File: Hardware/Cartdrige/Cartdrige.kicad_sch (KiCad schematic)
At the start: 3 parts, among them J2 PORT1, U1 28C256

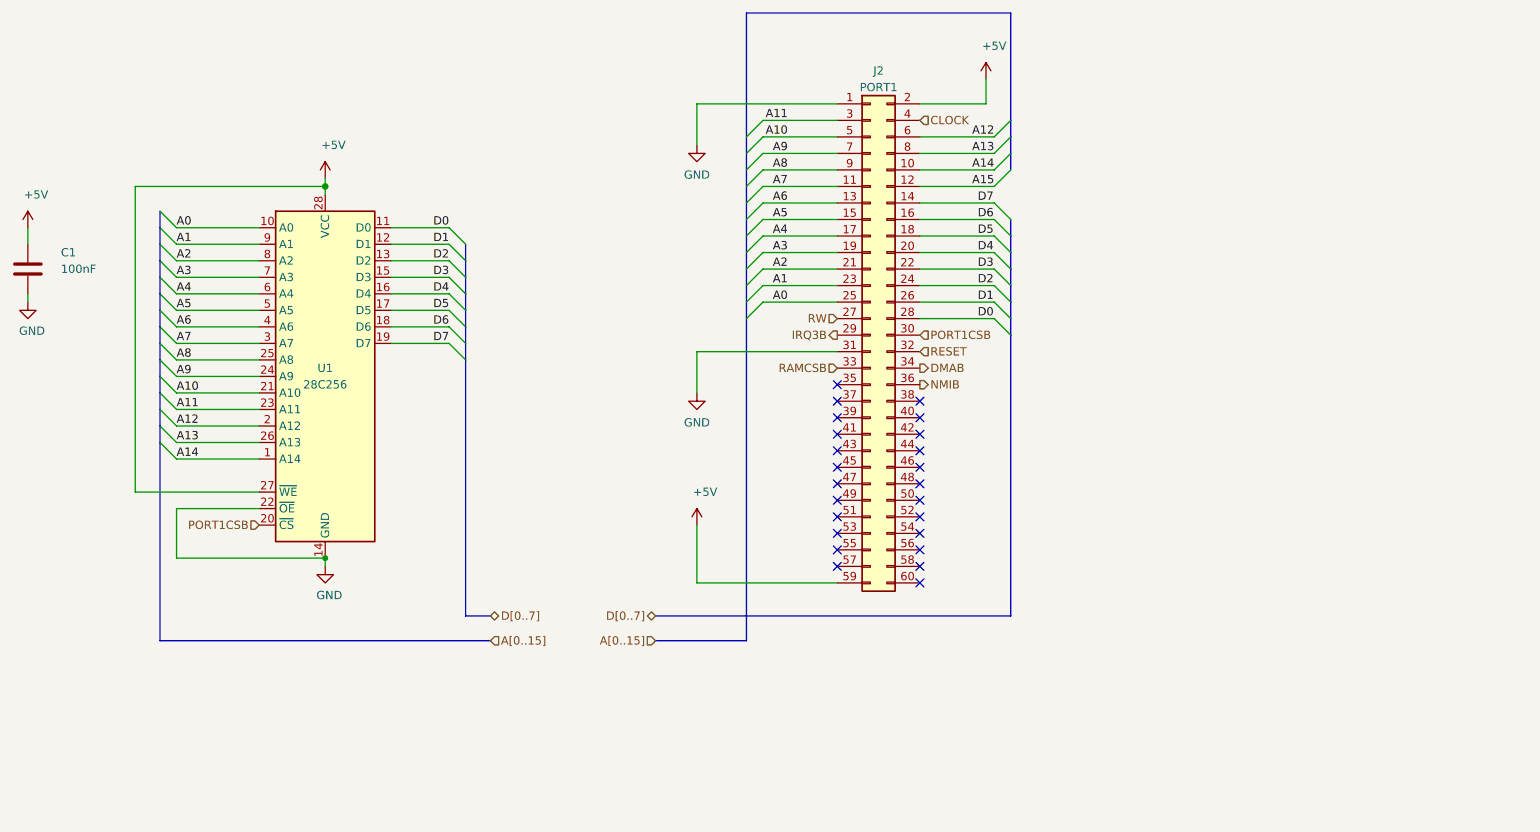
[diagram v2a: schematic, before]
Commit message: A lot of new hardware
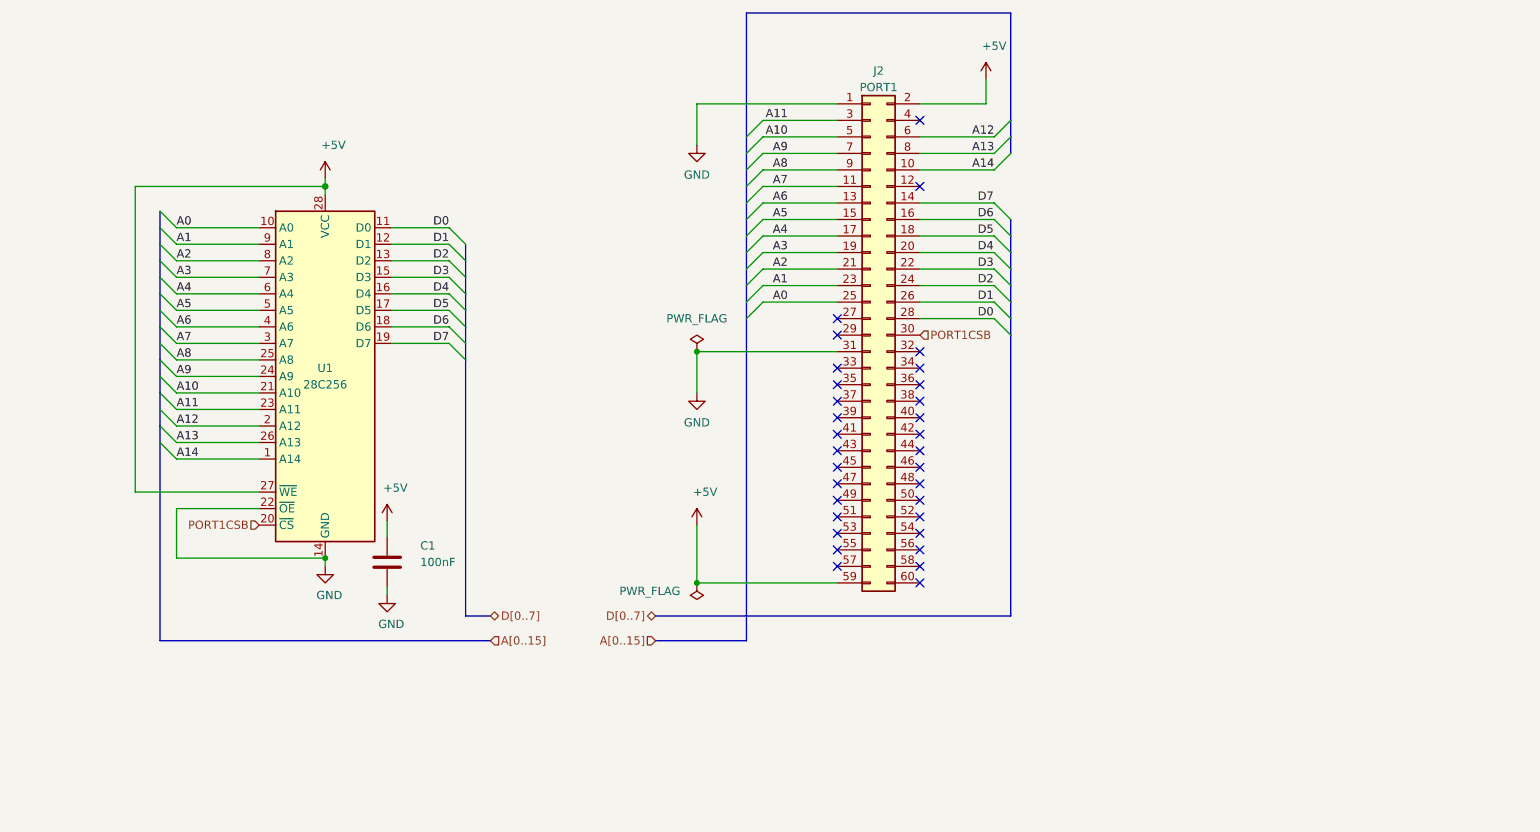
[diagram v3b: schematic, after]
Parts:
- J2: footprint NESConnector:NES_PCBEdge -> Connector_NES:NES_PCBEdge
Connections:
- net A15: no longer names the net of J2.12 (Pin_12)
- net CLOCK: no longer names the net of J2.4 (Pin_4)
- net DMAB: no longer names the net of J2.34 (Pin_34)
- net IRQ3B: no longer names the net of J2.29 (Pin_29)
- net NMIB: no longer names the net of J2.36 (Pin_36)
- net RAMCSB: no longer names the net of J2.33 (Pin_33)
- net RESET: no longer names the net of J2.32 (Pin_32)
- net RW: no longer names the net of J2.27 (Pin_27)
- no-connect marks 24 -> 32
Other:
- moved on the sheet: C1
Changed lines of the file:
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@@
   (junction (at 68.58 100.33) (diameter 0) (color 0 0 0 0)
+  )
+  (junction (at 125.73 68.58) (diameter 0) (color 0 0 0 0)
+  )
+  (junction (at 125.73 104.14) (diameter 0) (color 0 0 0 0)
   )
   (no_connect (at 160.02 96.52))
   (no_connect (at 160.02 101.6))
   (no_connect (at 160.02 91.44))
+  (no_connect (at 160.02 68.58))
   (no_connect (at 147.32 88.9))
   (no_connect (at 147.32 101.6))
   (no_connect (at 147.32 81.28))
+  (no_connect (at 160.02 43.18))
   (no_connect (at 147.32 83.82))
   (no_connect (at 147.32 76.2))
   (no_connect (at 160.02 86.36))
+  (no_connect (at 160.02 33.02))
+  (no_connect (at 160.02 71.12))
   (no_connect (at 160.02 88.9))
+  (no_connect (at 160.02 73.66))
+  (no_connect (at 147.32 71.12))
   (no_connect (at 160.02 93.98))
   (no_connect (at 160.02 104.14))
   (no_connect (at 147.32 96.52))
+  (no_connect (at 147.32 66.04))
   (no_connect (at 147.32 99.06))
   (no_connect (at 147.32 91.44))
@@
   (no_connect (at 147.32 73.66))
   (no_connect (at 160.02 76.2))
+  (no_connect (at 147.32 63.5))
   (no_connect (at 160.02 99.06))
   (no_connect (at 160.02 81.28))
@@
     (stroke (width 0.1524) (type solid))
   )
-  (bus_entry (at 173.99 40.64) (size -2.54 2.54)
-    (stroke (width 0.1524) (type solid))
-  )
   (bus_entry (at 43.18 52.07) (size 2.54 2.54)
     (stroke (width 0.1524) (type solid))
@@
     (stroke (width 0) (type solid))
   )
-  (wire (pts (xy 22.86 59.69) (xy 22.86 60.96))
+  (wire (pts (xy 78.105 104.775) (xy 78.105 106.045))
     (stroke (width 0) (type solid))
   )
@@
     (stroke (width 0) (type solid))
   )
-  (wire (pts (xy 171.45 43.18) (xy 160.02 43.18))
-    (stroke (width 0) (type solid))
-  )
   (wire (pts (xy 45.72 100.33) (xy 68.58 100.33))
     (stroke (width 0) (type default))
@@
     (stroke (width 0) (type solid))
   )
-  (bus (pts (xy 173.99 38.1) (xy 173.99 40.64))
-    (stroke (width 0) (type solid))
-  )
   (wire (pts (xy 135.89 45.72) (xy 147.32 45.72))
     (stroke (width 0) (type solid))
@@
     (stroke (width 0) (type default))
   )
-  (wire (pts (xy 22.86 49.53) (xy 22.86 52.07))
+  (wire (pts (xy 78.105 94.615) (xy 78.105 97.155))
     (stroke (width 0) (type solid))
   )
@@
     (effects (font (size 1.27 1.27)) (justify right bottom))
   )
-  (label "A15" (at 171.45 43.18 180) (fields_autoplaced)
-    (effects (font (size 1.27 1.27)) (justify right bottom))
-  )
   (label "A13" (at 45.72 82.55 0) (fields_autoplaced)
     (effects (font (size 1.27 1.27)) (justify left bottom))
+  )
+  (hierarchical_label "D[0..7]" (shape bidirectional) (at 93.98 109.22 0) (fields_autoplaced)
+    (effects (font (size 1.27 1.27)) (justify left))
   )
   (hierarchical_label "PORT1CSB" (shape input) (at 160.02 66.04 0) (fields_autoplaced)
     (effects (font (size 1.27 1.27)) (justify left))
   )
-  (hierarchical_label "RAMCSB" (shape input) (at 147.32 71.12 180) (fields_autoplaced)
-    (effects (font (size 1.27 1.27)) (justify right))
-  )
-  (hierarchical_label "D[0..7]" (shape bidirectional) (at 93.98 109.22 0) (fields_autoplaced)
-    (effects (font (size 1.27 1.27)) (justify left))
-  )
   (hierarchical_label "D[0..7]" (shape bidirectional) (at 119.38 109.22 180) (fields_autoplaced)
     (effects (font (size 1.27 1.27)) (justify right))
   )
-  (hierarchical_label "RW" (shape input) (at 147.32 63.5 180) (fields_autoplaced)
-    (effects (font (size 1.27 1.27)) (justify right))
-  )
   (hierarchical_label "A[0..15]" (shape input) (at 93.98 113.03 0) (fields_autoplaced)
     (effects (font (size 1.27 1.27)) (justify left))
   )
-  (hierarchical_label "CLOCK" (shape input) (at 160.02 33.02 0) (fields_autoplaced)
-    (effects (font (size 1.27 1.27)) (justify left))
-  )
-  (hierarchical_label "IRQ3B" (shape output) (at 147.32 66.04 180) (fields_autoplaced)
-    (effects (font (size 1.27 1.27)) (justify right))
-  )
-  (hierarchical_label "RESET" (shape input) (at 160.02 68.58 0) (fields_autoplaced)
-    (effects (font (size 1.27 1.27)) (justify left))
-  )
   (hierarchical_label "A[0..15]" (shape input) (at 119.38 113.03 180) (fields_autoplaced)
     (effects (font (size 1.27 1.27)) (justify right))
   )
-  (hierarchical_label "NMIB" (shape output) (at 160.02 73.66 0) (fields_autoplaced)
-    (effects (font (size 1.27 1.27)) (justify left))
-  )
-  (hierarchical_label "DMAB" (shape output) (at 160.02 71.12 0) (fields_autoplaced)
-    (effects (font (size 1.27 1.27)) (justify left))
-  )
   (hierarchical_label "PORT1CSB" (shape input) (at 58.42 95.25 180) (fields_autoplaced)
     (effects (font (size 1.27 1.27)) (justify right))
+  )
+  (symbol (lib_id "power:PWR_FLAG") (at 125.73 68.58 0) (unit 1)
+    (in_bom yes) (on_board yes) (dnp no) (fields_autoplaced)
+    (property "Reference" "#FLG02" (at 125.73 66.675 0)
+      (effects (font (size 1.27 1.27)) hide)
+    )
+    (property "Value" "PWR_FLAG" (at 125.73 63.5 0)
+      (effects (font (size 1.27 1.27)))
+    )
+    (property "Footprint" "" (at 125.73 68.58 0)
+      (effects (font (size 1.27 1.27)) hide)
+    )
+    (property "Datasheet" "~" (at 125.73 68.58 0)
+      (effects (font (size 1.27 1.27)) hide)
+    )
+    (pin "1")
+    (instances
+      (project "Cartdrige"
+        (path "/37e9d49f-81bc-4d5c-bab0-7c054d57d038"
+          (reference "#FLG02") (unit 1)
+        )
+      )
+    )
   )
   (symbol (lib_id "power:GND") (at 125.73 36.83 0) (mirror y) (unit 1)
@@
     )
     (property "Datasheet" "http://ww1.microchip.com/downloads/en/DeviceDoc/doc0006.pdf" (at 68.58 72.39 0)
+      (effects (font (size 1.27 1.27)) hide)
+    )
+    (property "Sim.Enable" "0" (at 68.58 72.39 0)
       (effects (font (size 1.27 1.27)) hide)
     )
@@
     )
   )
-  (symbol (lib_id "Device:C") (at 22.86 55.88 0) (unit 1)
+  (symbol (lib_id "Device:C") (at 78.105 100.965 0) (unit 1)
     (in_bom yes) (on_board yes) (dnp no)
-    (property "Reference" "C1" (at 27.94 53.34 0)
+    (property "Reference" "C1" (at 83.185 98.425 0)
       (effects (font (size 1.27 1.27)) (justify left))
     )
-    (property "Value" "100nF" (at 27.94 55.88 0)
+    (property "Value" "100nF" (at 83.185 100.965 0)
       (effects (font (size 1.27 1.27)) (justify left))
     )
-    (property "Footprint" "Capacitor_THT:C_Disc_D5.0mm_W2.5mm_P2.50mm" (at 23.8252 59.69 0)
-      (effects (font (size 1.27 1.27)) hide)
-    )
-    (property "Datasheet" "" (at 22.86 55.88 0)
+    (property "Footprint" "Capacitor_THT:C_Disc_D5.0mm_W2.5mm_P2.50mm" (at 79.0702 104.775 0)
+      (effects (font (size 1.27 1.27)) hide)
+    )
+    (property "Datasheet" "~" (at 78.105 100.965 0)
       (effects (font (size 1.27 1.27)) hide)
     )
@@
       (effects (font (size 1.27 1.27)))
     )
-    (property "Footprint" "NESConnector:NES_PCBEdge" (at 152.4 66.04 0)
+    (property "Footprint" "Connector_NES:NES_PCBEdge" (at 152.4 66.04 0)
       (effects (font (size 1.27 1.27)) hide)
     )
     (property "Datasheet" "~" (at 152.4 66.04 0)
+      (effects (font (size 1.27 1.27)) hide)
+    )
+    (property "Sim.Enable" "0" (at 152.4 66.04 0)
       (effects (font (size 1.27 1.27)) hide)
     )
@@
     )
   )
-  (symbol (lib_id "power:+5V") (at 22.86 49.53 0) (unit 1)
+  (symbol (lib_id "power:+5V") (at 78.105 94.615 0) (unit 1)
     (in_bom yes) (on_board yes) (dnp no)
-    (property "Reference" "#PWR03" (at 22.86 53.34 0)
-      (effects (font (size 1.27 1.27)) hide)
-    )
-    (property "Value" "+5V" (at 24.13 44.45 0)
-      (effects (font (size 1.27 1.27)))
-    )
-    (property "Footprint" "" (at 22.86 49.53 0)
-      (effects (font (size 1.27 1.27)) hide)
-    )
-    (property "Datasheet" "" (at 22.86 49.53 0)
+    (property "Reference" "#PWR03" (at 78.105 98.425 0)
+      (effects (font (size 1.27 1.27)) hide)
+    )
+    (property "Value" "+5V" (at 79.375 89.535 0)
+      (effects (font (size 1.27 1.27)))
+    )
+    (property "Footprint" "" (at 78.105 94.615 0)
+      (effects (font (size 1.27 1.27)) hide)
+    )
+    (property "Datasheet" "" (at 78.105 94.615 0)
       (effects (font (size 1.27 1.27)) hide)
     )
@@
     )
   )
-  (symbol (lib_id "power:GND") (at 22.86 60.96 0) (unit 1)
+  (symbol (lib_id "power:GND") (at 78.105 106.045 0) (unit 1)
     (in_bom yes) (on_board yes) (dnp no)
-    (property "Reference" "#PWR04" (at 22.86 67.31 0)
-      (effects (font (size 1.27 1.27)) hide)
-    )
-    (property "Value" "GND" (at 23.495 65.405 0)
-      (effects (font (size 1.27 1.27)))
-    )
-    (property "Footprint" "" (at 22.86 60.96 0)
-      (effects (font (size 1.27 1.27)) hide)
-    )
-    (property "Datasheet" "" (at 22.86 60.96 0)
+    (property "Reference" "#PWR04" (at 78.105 112.395 0)
+      (effects (font (size 1.27 1.27)) hide)
+    )
+    (property "Value" "GND" (at 78.74 110.49 0)
+      (effects (font (size 1.27 1.27)))
+    )
+    (property "Footprint" "" (at 78.105 106.045 0)
+      (effects (font (size 1.27 1.27)) hide)
+    )
+    (property "Datasheet" "" (at 78.105 106.045 0)
       (effects (font (size 1.27 1.27)) hide)
     )
@@
         )
       )
+    )
+  )
+  (symbol (lib_id "power:PWR_FLAG") (at 125.73 104.14 180) (unit 1)
+    (in_bom yes) (on_board yes) (dnp no) (fields_autoplaced)
+    (property "Reference" "#FLG01" (at 125.73 106.045 0)
+      (effects (font (size 1.27 1.27)) hide)
+    )
+    (property "Value" "PWR_FLAG" (at 123.19 105.41 0)
+      (effects (font (size 1.27 1.27)) (justify left))
+    )
+    (property "Footprint" "" (at 125.73 104.14 0)
+      (effects (font (size 1.27 1.27)) hide)
+    )
+    (property "Datasheet" "~" (at 125.73 104.14 0)
+      (effects (font (size 1.27 1.27)) hide)
+    )
+    (pin "1")
+    (instances
+      (project "Cartdrige"
+        (path "/37e9d49f-81bc-4d5c-bab0-7c054d57d038"
+          (reference "#FLG01") (unit 1)
+        )
+      )
